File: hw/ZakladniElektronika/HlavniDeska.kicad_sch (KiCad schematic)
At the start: 9 parts, among them SW1 SW_Push, SW2 SW_Push

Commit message: Hw wip
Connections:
- no-connect marks 3 -> 14
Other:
- removed sheet GPSKomunikacniModul
- sheet SpravceNapajeni ports: added OFF, USB_SEL, VUSB; removed 1V8, DSEL, EN_ALL, VBUS, VCC
- sheet USBPřepínač ports: added none; removed 3{USB}
- moved on the sheet: BZ1, D121, R27, R28, R37, R38, R39, SW1, SW2

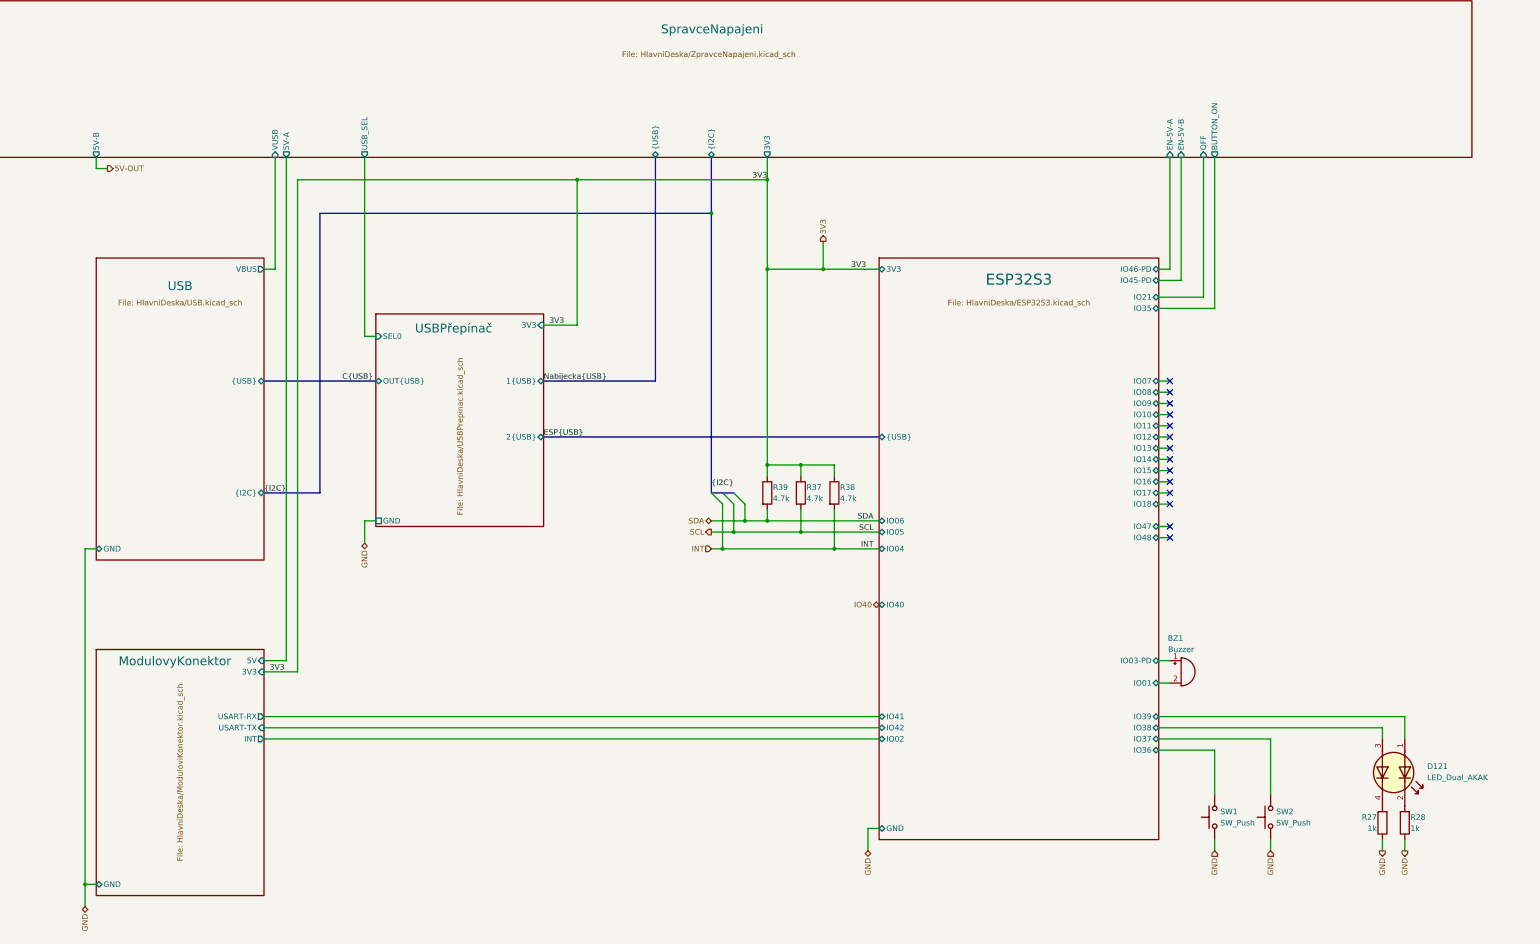
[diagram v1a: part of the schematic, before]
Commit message: Hw PCB
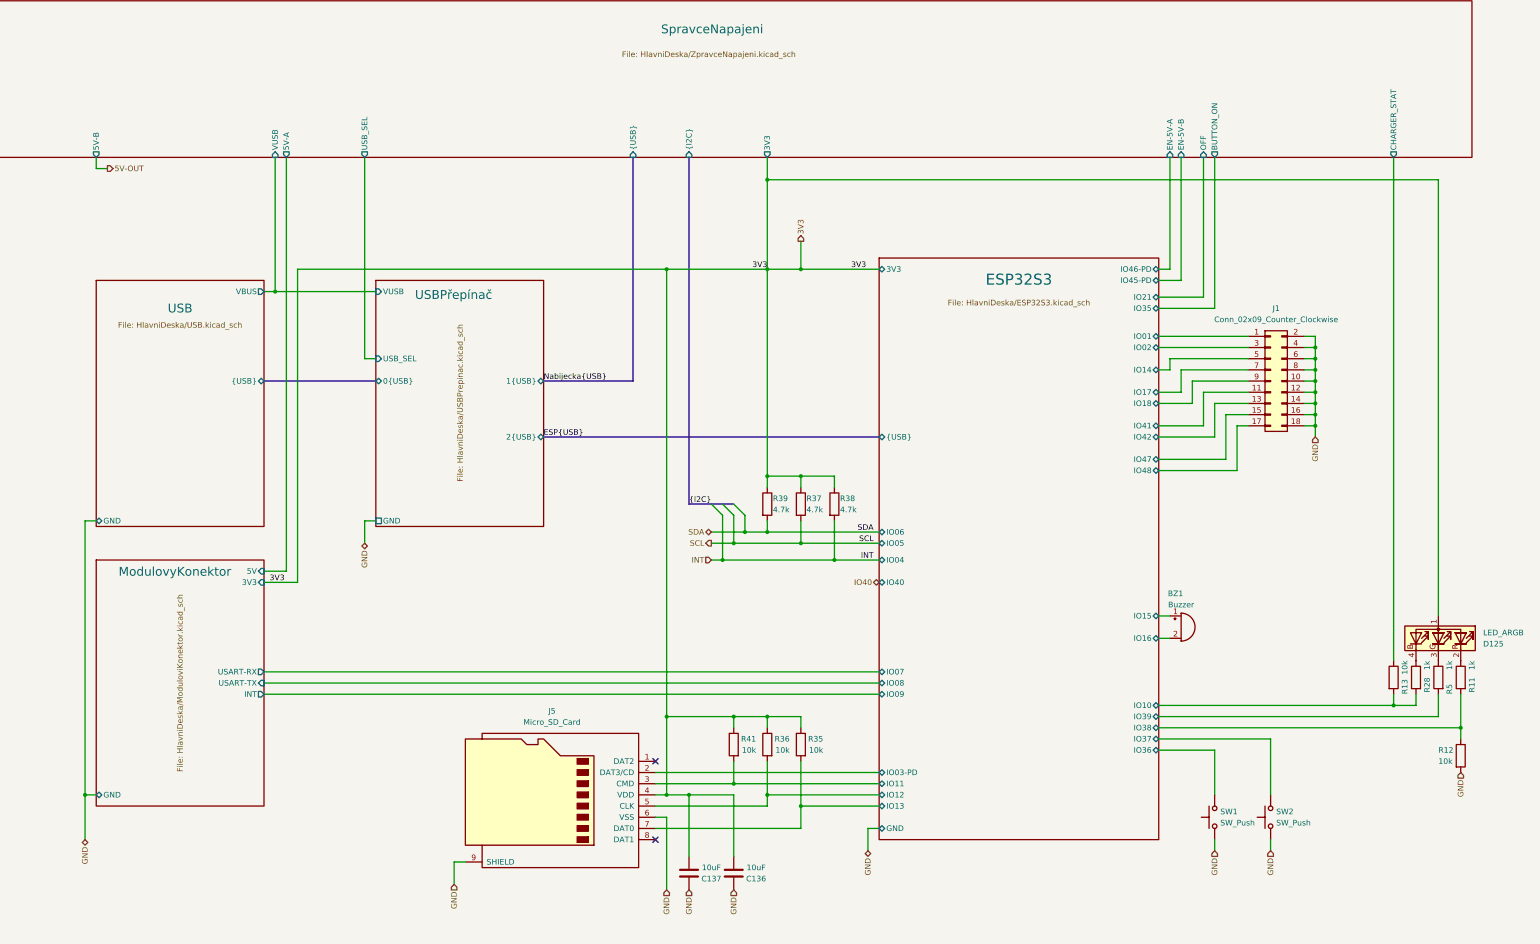
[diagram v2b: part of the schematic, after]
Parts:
- removed D121: LED_Dual_AKAK, RKL-LED:SMD,1.5x3.2mm 4pin, symbol Device:LED_Dual_AKAK
- removed R27: 1k, Resistor_SMD:R_0402_1005Metric, symbol Device:R
- added C136, C137: 10uF, Capacitor_SMD:C_0603_1608Metric, symbol Device:C
- added D125: LED_ARGB, RKL-LED:XL-3806RGBC-4L, symbol Device:LED_ARGB
- added J1: Conn_02x09_Counter_Clockwise, Connector_PinHeader_2.54mm:PinHeader_2x09_P2.54mm_Vertical, symbol Connector_Generic:Conn_02x09_Odd_Even
- added J5: Micro_SD_Card, Connector_Card:microSD_HC_Molex_47219-2001, symbol Connector:Micro_SD_Card
- added R11, R5: 1k, Resistor_SMD:R_0402_1005Metric, symbol Device:R
- added R12, R13, R35, R36, R41: 10k, Resistor_SMD:R_0402_1005Metric, symbol Device:R
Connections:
- net 3V3: now also C136.1, C137.1, D125.1 (A), J5.4 (VDD), R35.1, R36.1, R41.1
- net ESP32S3/IO01: now also J1.1 (Pin_1); no longer BZ1.2 (+)
- net ESP32S3/IO02: now also J1.3 (Pin_3)
- net ESP32S3/IO03-PD: now also J5.2 (DAT3/CD); no longer BZ1.1 (-)
- net ESP32S3/IO10: now also R28.2, R13.2
- net ESP32S3/IO11: now also J5.3 (CMD), R41.2
- net ESP32S3/IO12: now also J5.5 (CLK), R36.2
- net ESP32S3/IO13: now also J5.7 (DAT0), R35.2
- net ESP32S3/IO14: now also J1.5 (Pin_5)
- net ESP32S3/IO15: now also BZ1.1 (-)
- net ESP32S3/IO16: now also BZ1.2 (+)
- net ESP32S3/IO17: now also J1.7 (Pin_7)
- net ESP32S3/IO18: now also J1.9 (Pin_9)
- net ESP32S3/IO38: now also R11.2, R12.1
- net ESP32S3/IO39: now also R5.2
- net ESP32S3/IO41: now also J1.11 (Pin_11)
- net ESP32S3/IO42: now also J1.13 (Pin_13)
- net ESP32S3/IO47: now also J1.15 (Pin_15)
- net ESP32S3/IO48: now also J1.17 (Pin_17)
- net GND: now also C136.2, C137.2, J1.10 (Pin_10), J1.12 (Pin_12), J1.14 (Pin_14), J1.16 (Pin_16), J1.18 (Pin_18), J1.2 (Pin_2), J1.4 (Pin_4), J1.6 (Pin_6), J1.8 (Pin_8), J5.6 (VSS), J5.9 (SHIELD), R12.2; no longer R28.1
- new net: D125.4 (BK), R28.1
- new net: D125.2 (RK), R11.1
- new net: D125.3 (GK), R5.1
- new net SpravceNapajeni/CHARGER_STAT: R13.1
- no-connect marks 14 -> 2
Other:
- sheet SpravceNapajeni ports: added CHARGER_STAT; removed none
- sheet USB ports: added none; removed {I2C}
- sheet USBPřepínač ports: added 0{USB}, USB_SEL, VUSB; removed 3V3, OUT{USB}, SEL0
- moved on the sheet: BZ1, R28, R37, R38, R39
